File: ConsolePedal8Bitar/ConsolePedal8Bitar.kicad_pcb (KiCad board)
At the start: 2 copper layers, 100 x 60 mm, 27 parts, among them IC1 CD4069UBE, J1 Conn_02x25_Counter_Clockwise, Q1 2N3904

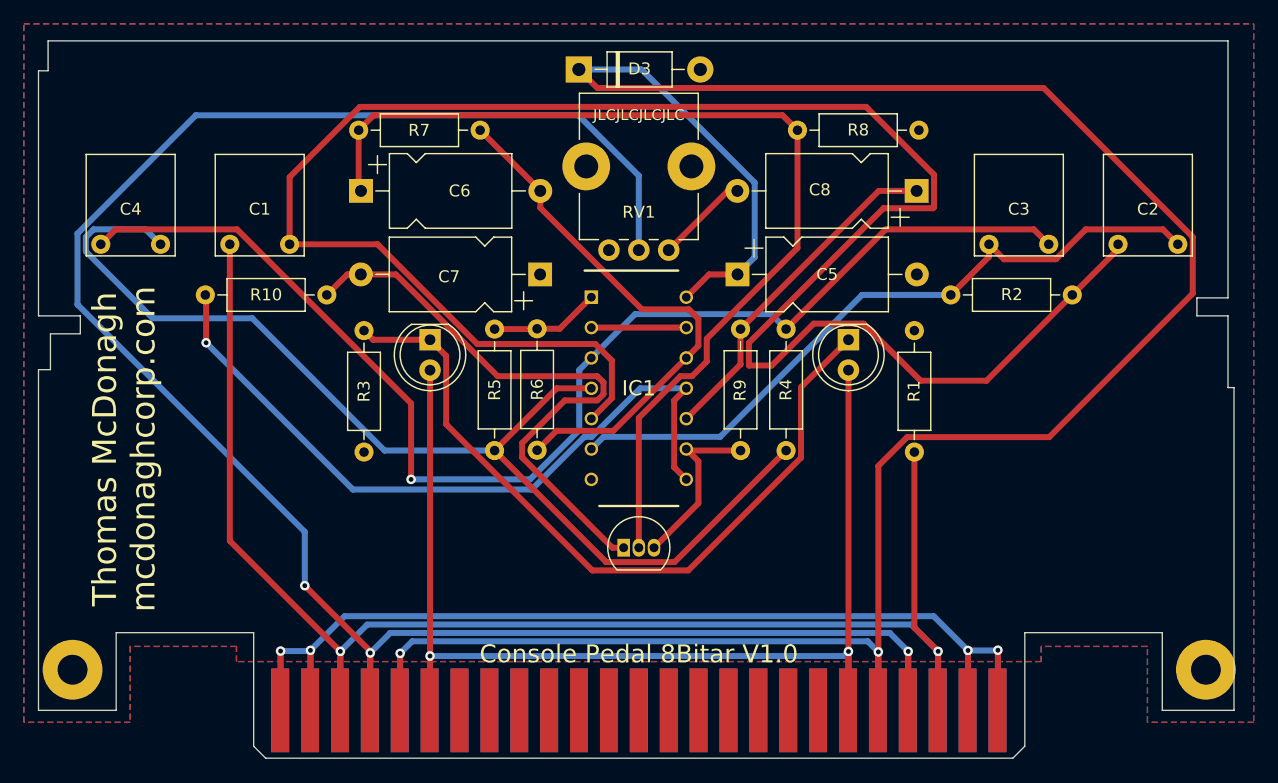
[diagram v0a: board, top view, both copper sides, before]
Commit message: Finalized and plotted new version
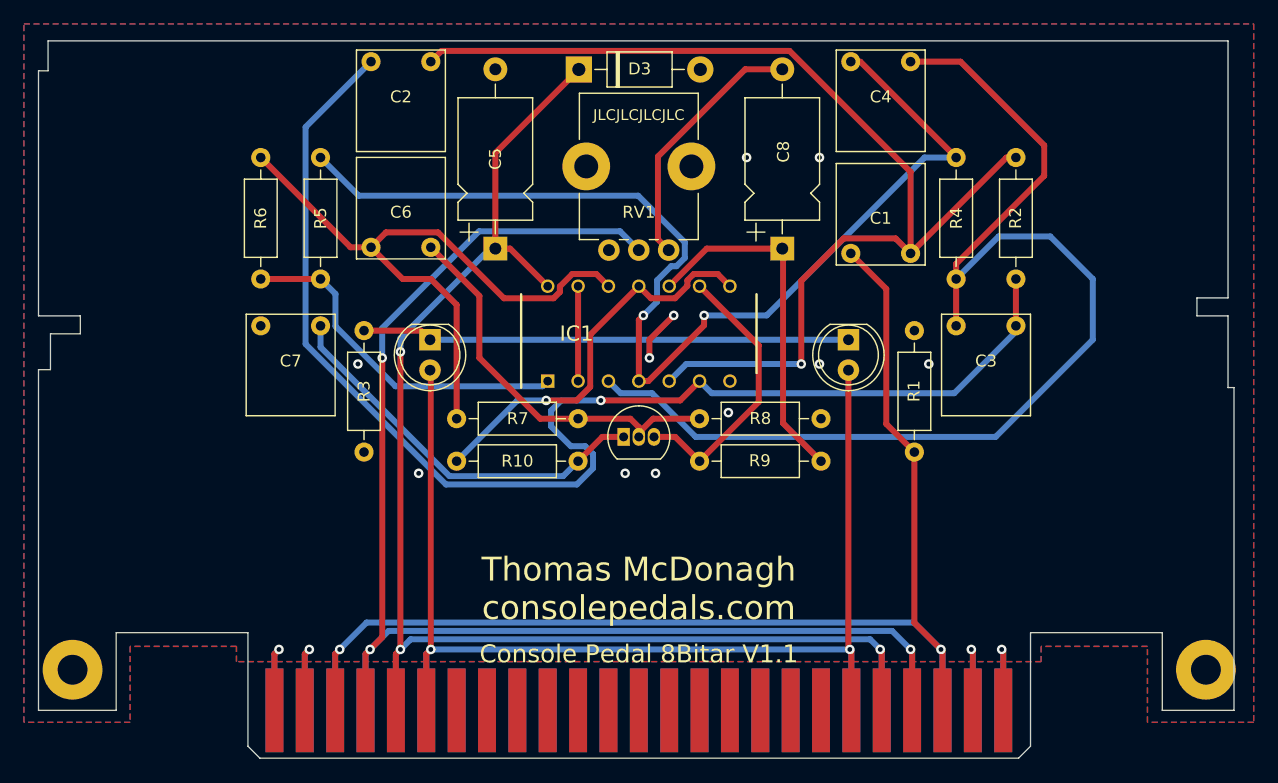
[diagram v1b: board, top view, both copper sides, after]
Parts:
- C6, C7: footprint Capacitor_THT:CP_Axial_L10.0mm_D6.0mm_P15.00mm_Horizontal -> libraries:C_Flat_L7.2_H6.5
- J1: footprint libraries:N64-Connector -> libraries:N64-Connector-Wide
- moved C2 69.0 mm to (110.3, 72.1), turned to 0 degrees
- moved C4 59.5 mm to (150.4, 72.1), turned to 0 degrees
- moved C1 51.9 mm to (155.4, 87.4)
- moved R6 33.7 mm to (101.1, 79.8), turned to 270 degrees
- moved R4 28.3 mm to (159.3, 79.8), turned to 270 degrees
- moved R8 25.5 mm to (137.8, 101.6)
- moved R10 25.2 mm to (127.6, 105.2)
- moved R7 24.2 mm to (117.5, 101.6), turned to 0 degrees
- moved C7 23.8 mm to (101.1, 94.2), turned to 0 degrees
- moved C5 20.4 mm to (120.7, 87.4), turned to 90 degrees
- moved R5 15.1 mm to (106.1, 89.9), turned to 90 degrees
- moved R9 12.9 mm to (148.0, 105.2), turned to 180 degrees
- moved C8 12.2 mm to (144.7, 87.4), turned to 90 degrees
- moved C3 10.9 mm to (159.3, 94.2), turned to 0 degrees
- moved Q1 9.27 mm to (131.4, 103.1)
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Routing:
- net +9V: track 201.8 -> 122.3 mm, vias 2 -> 3
- net /pin5: track 164.9 -> 93.4 mm, vias 0 -> 1
- net GND: track 102.5 -> 46.0 mm, vias 4 -> 15
- net Net-(C6-Pad1): track 83.9 -> 33.4 mm
- net /pin6: track 58.8 -> 109.2 mm, vias 0 -> 1
- net /Output: track 170.4 -> 120.1 mm
- net /pin11: track 61.2 -> 33.4 mm
- net Net-(D1-Pad1): track 64.2 -> 40.8 mm
- net /pin1: track 9.20 -> 29.5 mm
- net /Input: track 127.0 -> 109.2 mm
- net Net-(C7-Pad2): track 49.9 -> 33.0 mm
- net Net-(C8-Pad2): track 7.79 -> 21.6 mm
- net /pin12: track 45.0 -> 55.2 mm
- net /pin9: track 14.8 -> 23.4 mm
- net /pin3: track 105.4 -> 97.5 mm, vias 1 -> 0
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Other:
- outline, holes or cut-outs redrawn
- board text added: "Console Pedal 8Bitar V1.1"
- board text added: "Thomas McDonagh consolepedals.com"
- board text removed: "Console Pedal 8Bitar V1.0"
- board text removed: "Thomas McDonagh mcdonaghcorp.com"
